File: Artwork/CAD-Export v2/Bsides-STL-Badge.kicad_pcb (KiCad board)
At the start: 2 copper layers, 94.9 x 137 mm, 7 parts

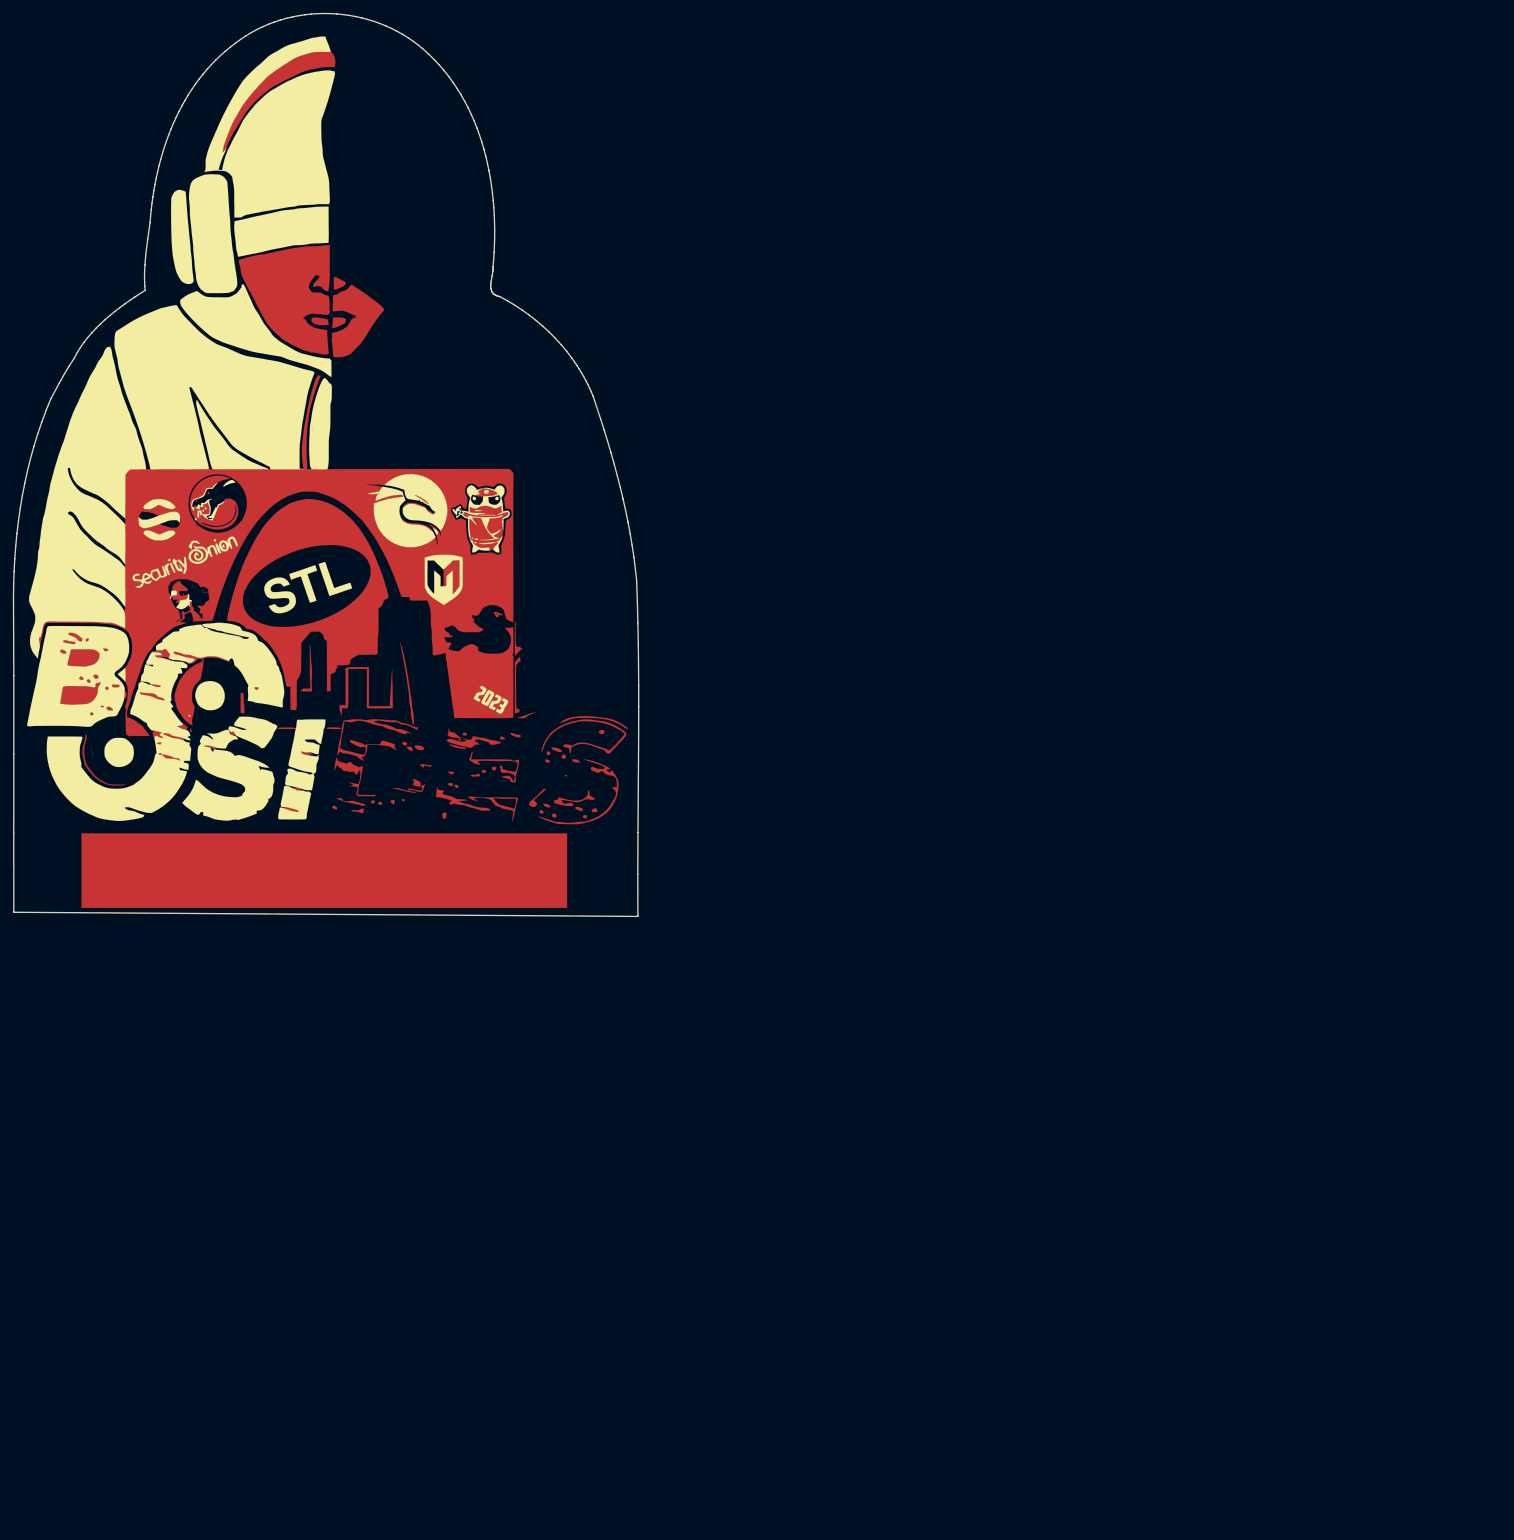
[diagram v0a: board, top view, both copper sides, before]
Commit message: Gerbers
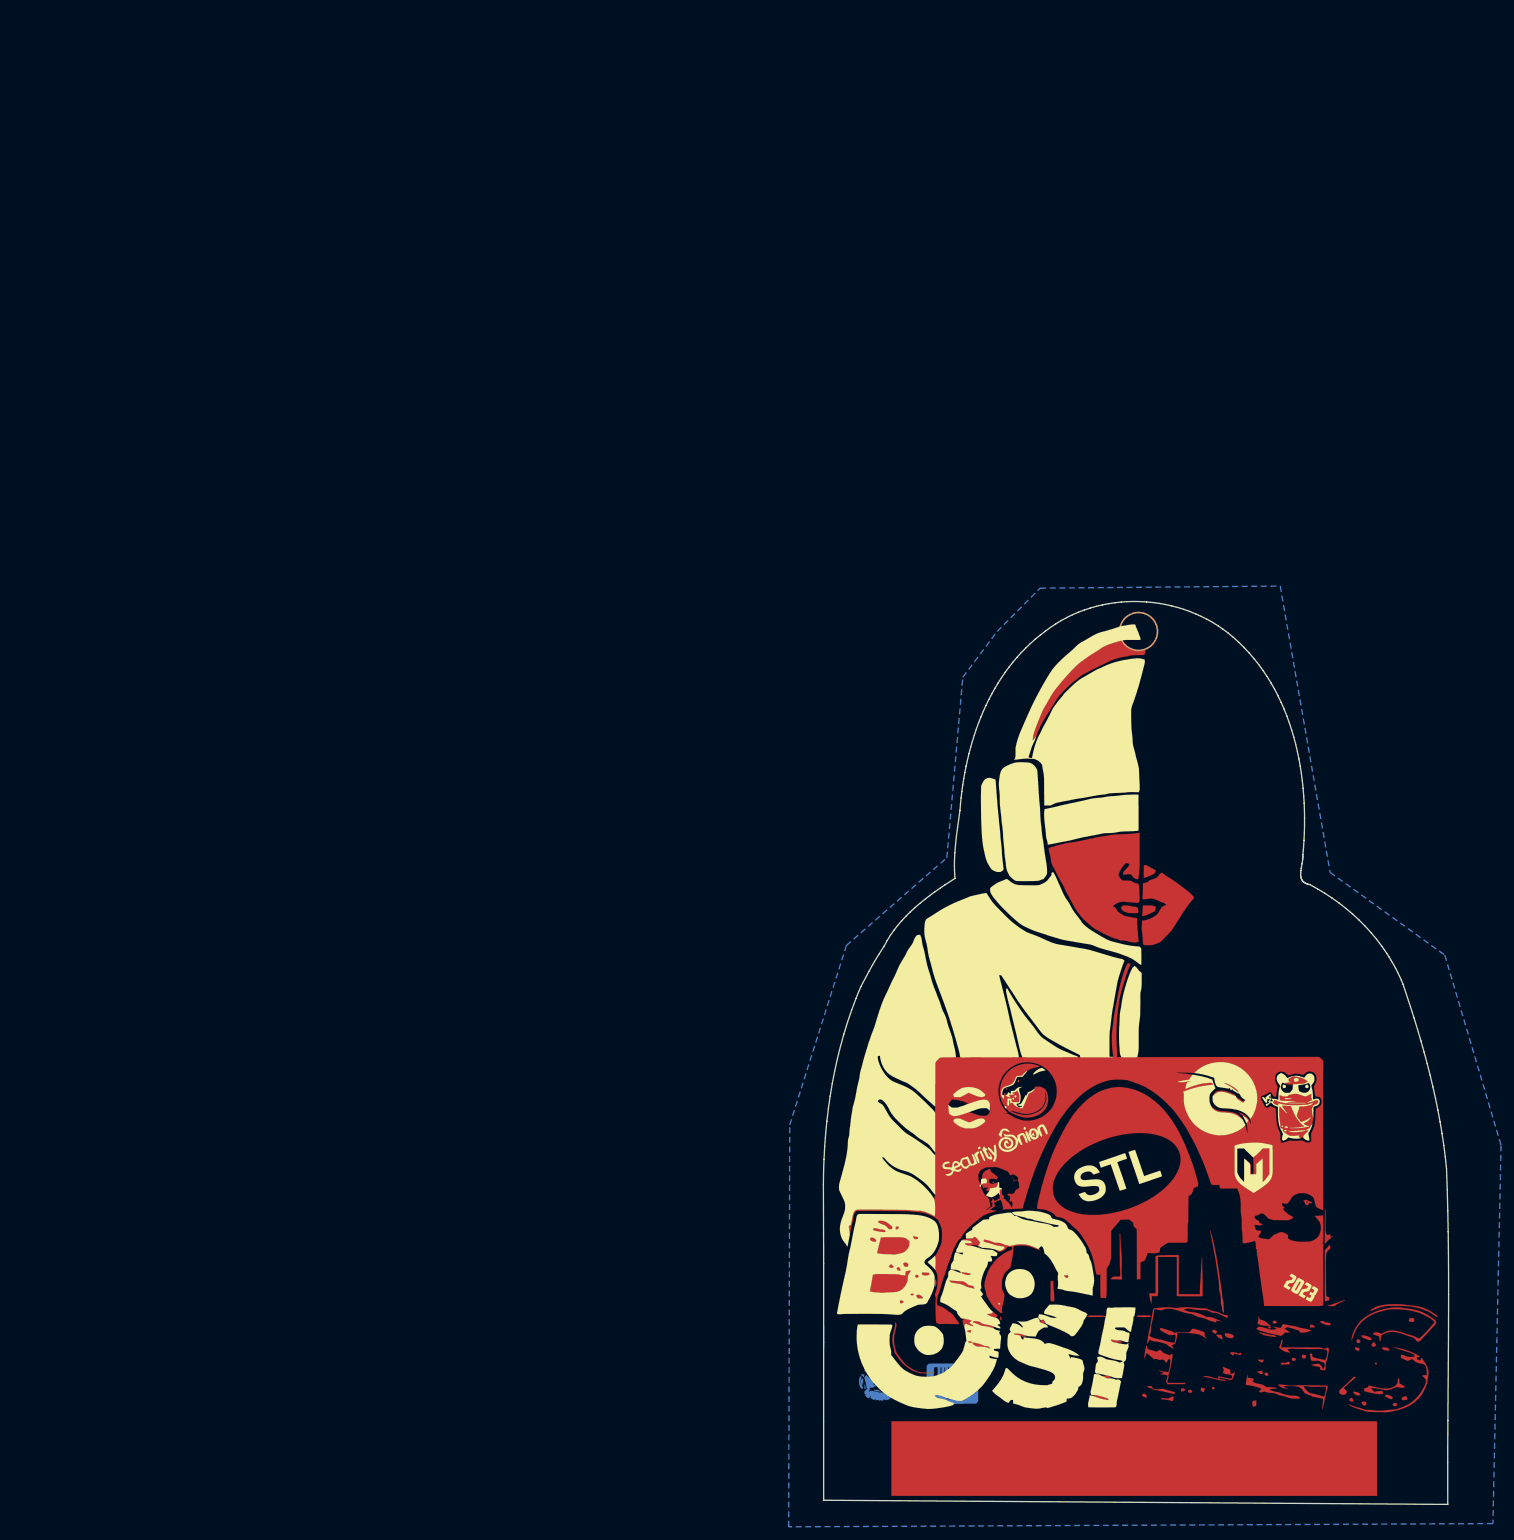
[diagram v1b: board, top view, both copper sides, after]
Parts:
- removed the G*** at (0.00, 0.00) (x7)
- added G*** (x7): LOGO, LOGO, F.Cu at (122.9, 89.2)
- added G***: LOGO, BadgePiratesLogos:BadgePiratesURL_B.SLK, F.Cu at (107.3, 103.1)
- added G***: NG_BSilk_B.Cu, BadgePiratesLogos:NG_B.Cu, F.Cu at (100.4, 137.6)
- added G***: BP Logo, BadgePiratesLogos:BPSkull_Distressed_B.SILK, F.Cu at (107.5, 94.1)
- added G***: fg, BadgePiratesLogos:FG_B.Cu, F.Cu at (89.7, 136.9)
- added REF**: 5.5mm, BadgePirates:Hole_5.5mm, F.Cu at (128.8, 23.7)
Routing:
- added copper zone on B.Cu, net (none)
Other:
- outline, holes or cut-outs redrawn
- net class Default removed
